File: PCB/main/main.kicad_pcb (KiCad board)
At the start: 2 copper layers, 100 x 100 mm, 46 parts, among them J1 Conn_01x33_Female, J2 Conn_01x33_Female, J3 Conn_01x33_Female, J4 Conn_01x33_Female, J5 USB_B_Micro, Q1 2N2222A, SW1 C13828, SW2 C13828, U1 TP4054, U2 MT3608L

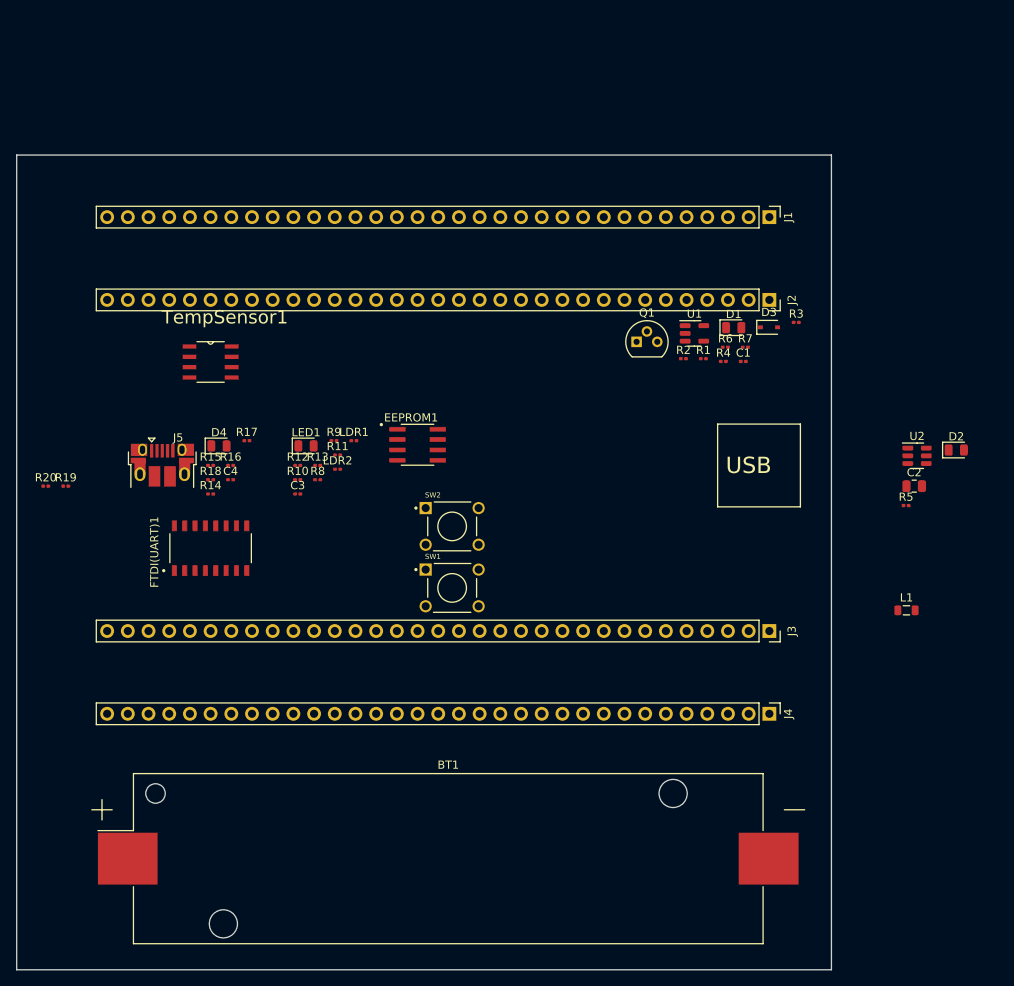
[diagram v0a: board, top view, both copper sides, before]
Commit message: updated gerbers and finalized PCB
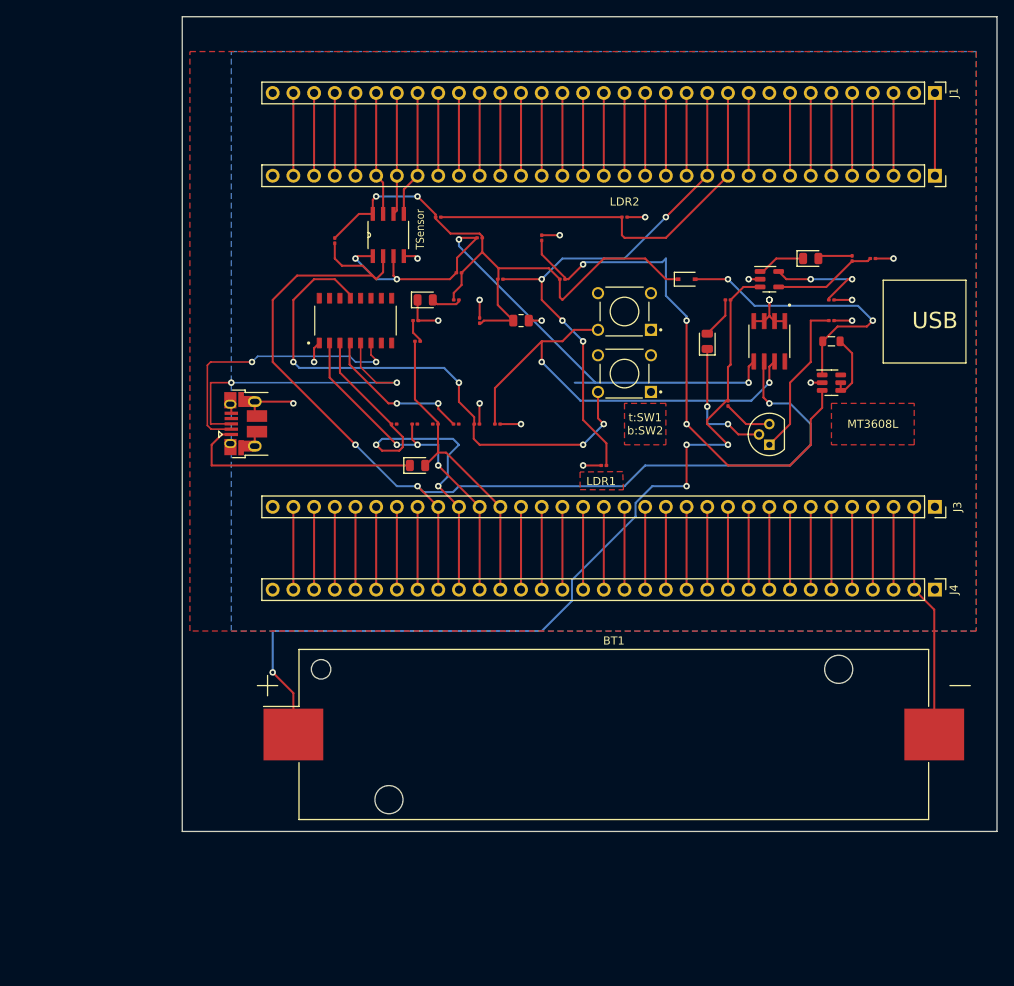
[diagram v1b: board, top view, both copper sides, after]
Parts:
- C4: value CT41G-0402-2X1-16V-0.1μF-K(N) -> 0.1μF
- R1: value 1650 -> 1800
- R3: value 100 -> 100ohms
- R5: value 1000 -> 1200
- moved C2 52.4 mm to (149.9, 78.7)
- moved LDR2 46.9 mm to (162.6, 66.0)
- moved R20 45.9 mm to (136.8, 91.4)
- moved EEPROM1 45.0 mm to (180.3, 81.3), turned to -90 degrees
- moved R19 41.0 mm to (134.3, 91.4)
- moved SW1 40.0 mm to (162.6, 77.6), turned to 180 degrees
- moved R14 36.2 mm to (147.0, 91.4)
- moved L1 34.3 mm to (188.0, 81.3), turned to 180 degrees
- moved R18 33.4 mm to (144.4, 91.4)
- moved R8 33.3 mm to (147.3, 73.7)
- moved FTDI(UART)1 33.1 mm to (129.5, 78.7)
- moved R10 32.2 mm to (142.2, 72.9), turned to 180 degrees
- moved R11 31.8 mm to (144.8, 68.6), turned to 180 degrees
- moved R5 31.0 mm to (190.5, 71.1), turned to -90 degrees
- moved C3 30.8 mm to (144.8, 78.7), turned to 90 degrees
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- renumbered TempSensor1 to TSensor
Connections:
- FTDI(UART)1 pad 15: +5V -> unconnected-(FTDI(UART)1-Pad15)
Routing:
- net /PA8: track 0.00 -> 135.9 mm, vias 0 -> 3
- net Net-(BT1-Pad1): track 0.00 -> 109.0 mm, vias 0 -> 4
- net GND: track 0.00 -> 80.3 mm, vias 0 -> 19
- net /Sensing/I2CBUS: track 0.00 -> 76.2 mm, vias 0 -> 4
- net /Power/Output: track 0.00 -> 75.3 mm, vias 0 -> 2
- net Net-(FTDI(UART)1-Pad13): track 0.00 -> 67.5 mm, vias 0 -> 4
- net /PC1: track 0.00 -> 66.6 mm, vias 0 -> 4
- net Net-(R6-Pad2): track 0.00 -> 66.6 mm, vias 0 -> 3
- net /microcontroller_interfacing/EEPROM MODE TP: track 0.00 -> 56.3 mm, vias 0 -> 2
- net /PC0: track 0.00 -> 50.9 mm
- net /PA9: track 0.00 -> 50.4 mm, vias 0 -> 2
- net /PA10: track 0.00 -> 43.7 mm, vias 0 -> 3
- net USB D+: track 0.00 -> 38.7 mm, vias 0 -> 2
- net /PA11: track 0.00 -> 37.6 mm
- net Net-(D3-Pad2): track 0.00 -> 35.3 mm, vias 0 -> 2
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- added copper zone on F.Cu, net +5V
- added copper zone on B.Cu, net GND
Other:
- board text added: "MT3608L"
- board text added: "t:SW1 b:SW2"
